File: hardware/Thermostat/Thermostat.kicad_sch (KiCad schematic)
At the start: 51 parts, among them J1 Barrel_Jack_Switch, J2 Conn_01x02_Pin, J3 AVR-ISP-6, J4 MainConnectorr, K1 G6E, K2 G6E, K3 G6E, K4 G6E, SW1 12MM, SW2 12MM, SW3 12MM, SW4 DIP-1, SW5 SW_Push, U1 GU112X16G-7003BL, U2 47L04, U4 UA78M05QDCYRQ1, U5 ATmega88-20A, U6 TMP116xxDRV, U8 DS1307Z+, Y1 Crystal, Y2 Crystal_GND23

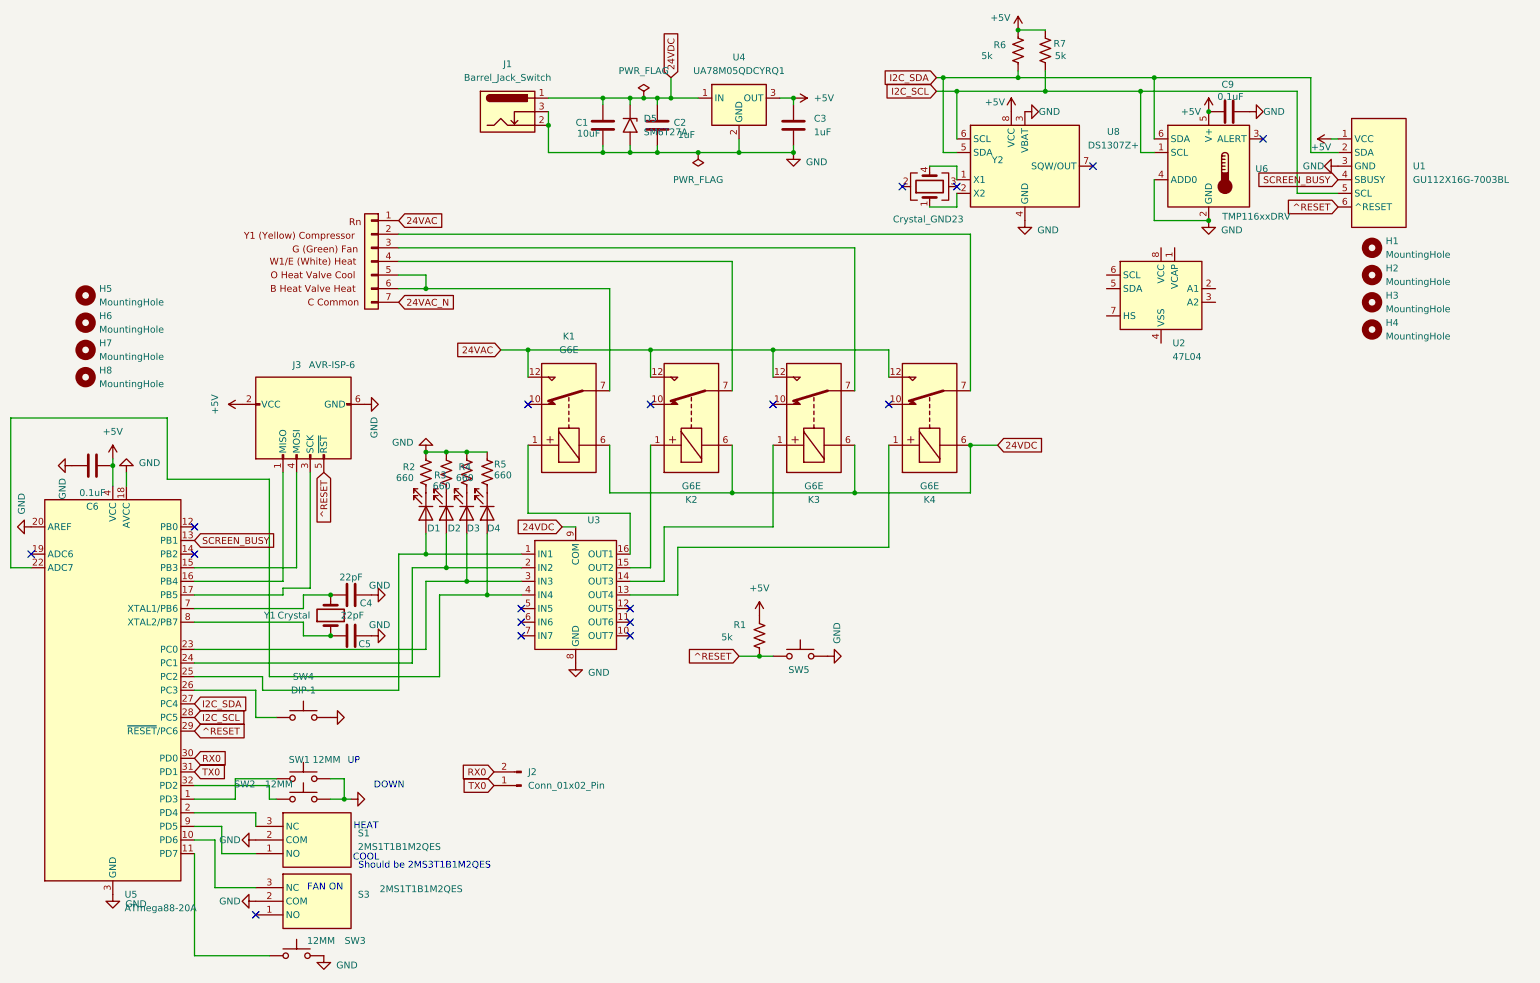
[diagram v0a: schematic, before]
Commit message: WIP
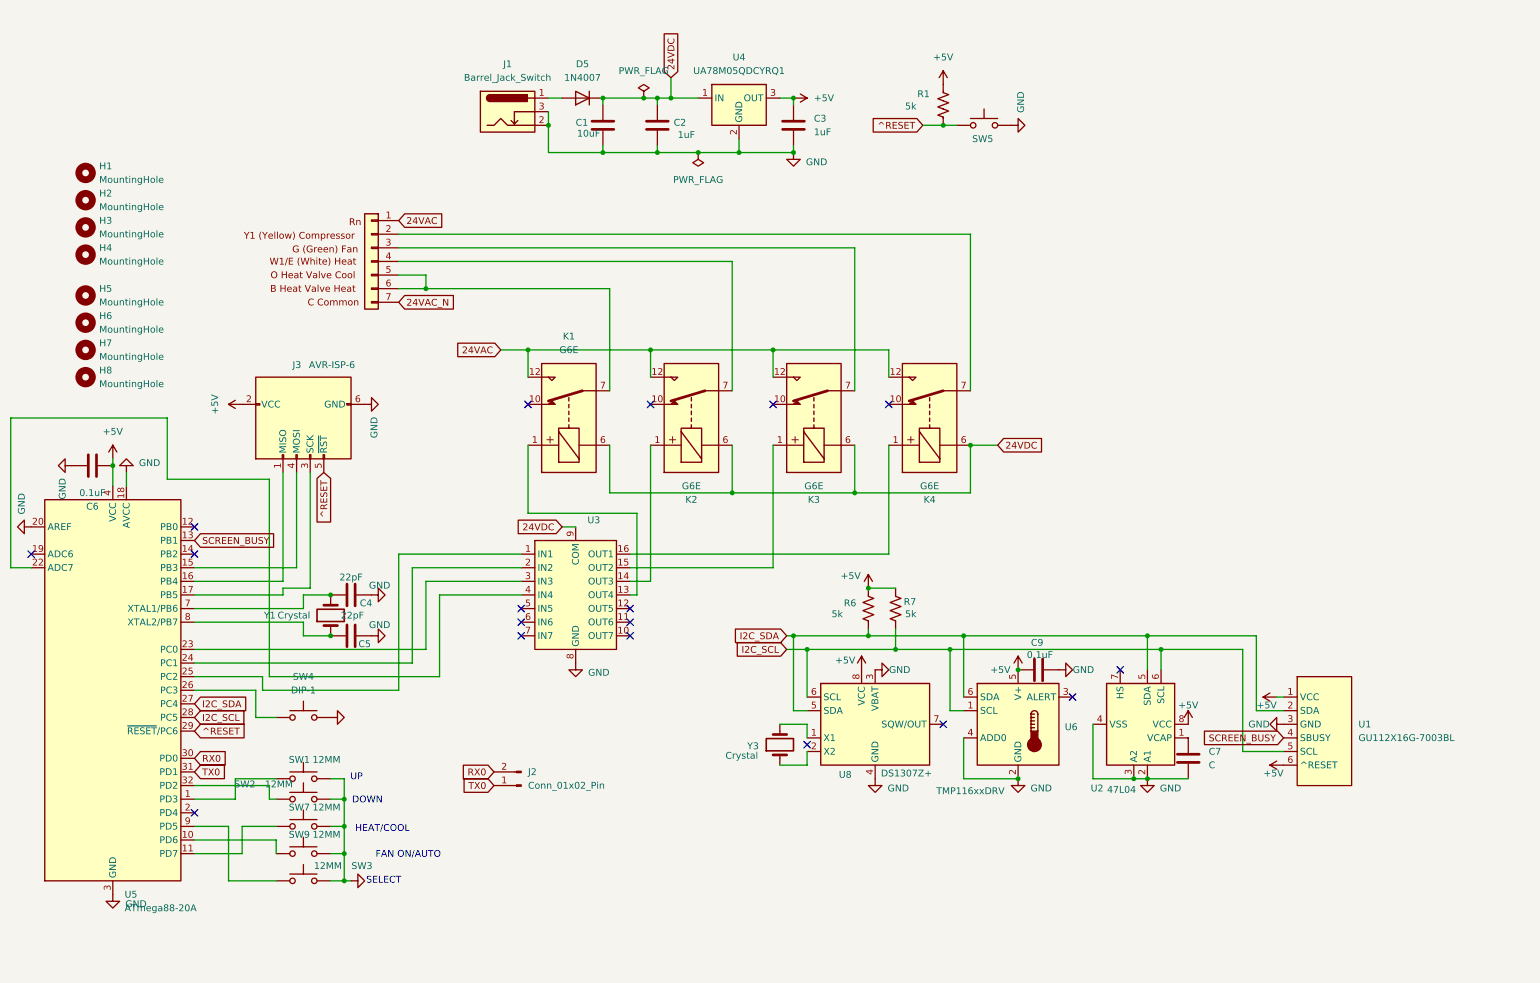
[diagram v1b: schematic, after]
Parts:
- removed D1, D2, D3, D4: LED, LED_SMD:LED_0805_2012Metric, symbol Device:LED
- removed D5: SM6T27A, Diode_SMD:D_SMB, symbol Diode:SM6T27A
- removed R2, R3, R4, R5: 660, Resistor_SMD:R_0603_1608Metric, symbol Device:R_US
- removed S1: 2MS1T1B1M2QES, ThermostatFootprints:2MS1T1B1M2QES, symbol ThermoSymbols:2MS3T1B1M2QES
- removed S3: 2MS1T1B1M2QES, ThermostatFootprints:2MS1T1B1M2QES, symbol ThermoSymbols:2MS1T1B1M2QES
- removed Y2: Crystal_GND23, Crystal:Crystal_SMD_5032-2Pin_5.0x3.2mm, symbol Device:Crystal_GND23
- added C7: C, Capacitor_SMD:C_0603_1608Metric, symbol Device:C
- added D5: 1N4007, Diode_THT:D_DO-41_SOD81_P10.16mm_Horizontal, symbol Diode:1N4007
- added SW7, SW9: 12MM, ThermostatFootprints:B3F, symbol Switch:SW_Push
- added Y3: Crystal, Crystal:Crystal_SMD_5032-2Pin_5.0x3.2mm, symbol Device:Crystal
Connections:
- net +5V: now also U1.6 (^RESET), U2.8 (VCC)
- net 24VDC: now also D5.1 (K); no longer J1.1
- net GND: now also U2.2 (A1), U2.3 (A2), U2.4 (VSS), C7.2, SW7.2, SW9.2
- net I2C_SCL: now also U2.6 (SCL)
- net I2C_SDA: now also U2.5 (SDA)
- net ^RESET: no longer U1.6 (^RESET)
- net at U8.1 (X1): now also Y3.2
- net at U8.2 (X2): now also Y3.1
- net at SW3.1: now also U5.9 (PD5); no longer U5.11 (PD7)
- net at U2.1 (VCAP): now also C7.1
- net at U5.10 (PD6): now also SW9.1
- net at K1.1: now also U3.13 (OUT4); no longer U3.16 (OUT1)
- net at K2.1: now also U3.14 (OUT3); no longer U3.15 (OUT2)
- net at K3.1: now also U3.15 (OUT2); no longer U3.14 (OUT3)
- net at K4.1: now also U3.16 (OUT1); no longer U3.13 (OUT4)
- new net: D5.2 (A), J1.1
- new net: SW7.1, U5.11 (PD7)
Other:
- note added: "FAN ON/AUTO"
- note added: "HEAT/COOL"
- note added: "SELECT"
- note removed: "COOL"
- note removed: "FAN ON"
- note removed: "HEAT"
- note removed: "Should be 2MS3T1B1M2QES"
- moved on the sheet: C9, H1, H2, H3, H4, R1, R6, R7, SW3, SW5, U1, U2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

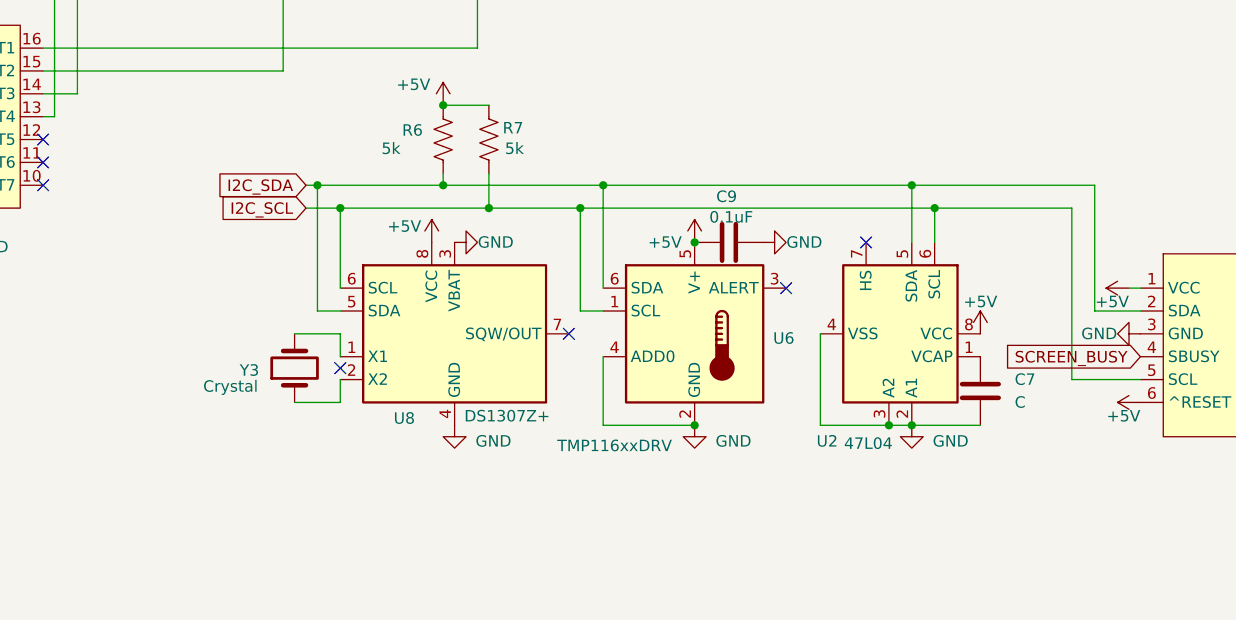
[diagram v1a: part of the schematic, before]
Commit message: WIP
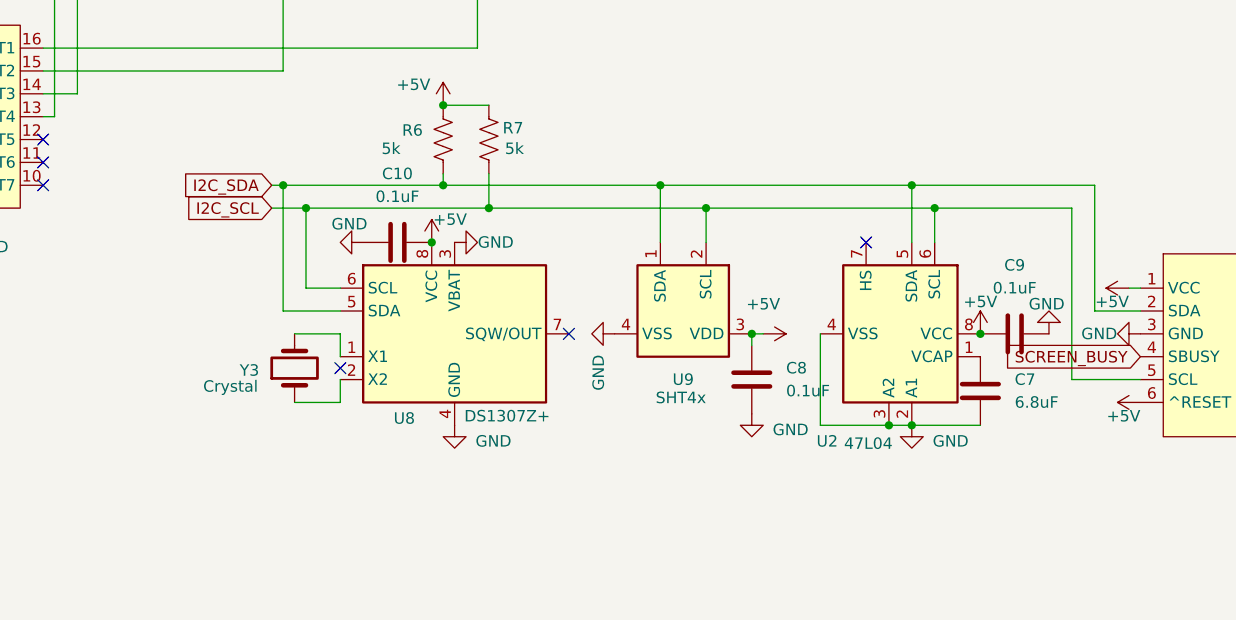
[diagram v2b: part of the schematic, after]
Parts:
- removed U6: TMP116xxDRV, Package_SON:WSON-6-1EP_2x2mm_P0.65mm_EP1x1.6mm_ThermalVias, symbol Sensor_Temperature:TMP116xxDRV
- added C10, C8: 0.1uF, Capacitor_SMD:C_0603_1608Metric, symbol Device:C
- added U9: SHT4x, Sensor_Humidity:Sensirion_DFN-4_1.5x1.5mm_P0.8mm_SHT4x_NoCentralPad, symbol Sensor_Humidity:SHT4x
- C7: value C -> 6.8uF
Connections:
- net +5V: now also C9.2, C10.1, C8.2, U9.3 (VDD); no longer C9.1
- net GND: now also C9.1, C10.2, C8.1, U9.4 (VSS); no longer C9.2
- net I2C_SCL: now also U9.2 (SCL)
- net I2C_SDA: now also U9.1 (SDA)
- no-connect marks 18 -> 17
